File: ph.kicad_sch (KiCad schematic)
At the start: 46 parts, among them J4 Conn_01x04_Pin, J5 Conn_Coaxial, J6 Conn_01x04_Pin, U17 CA3140, U18 TL081

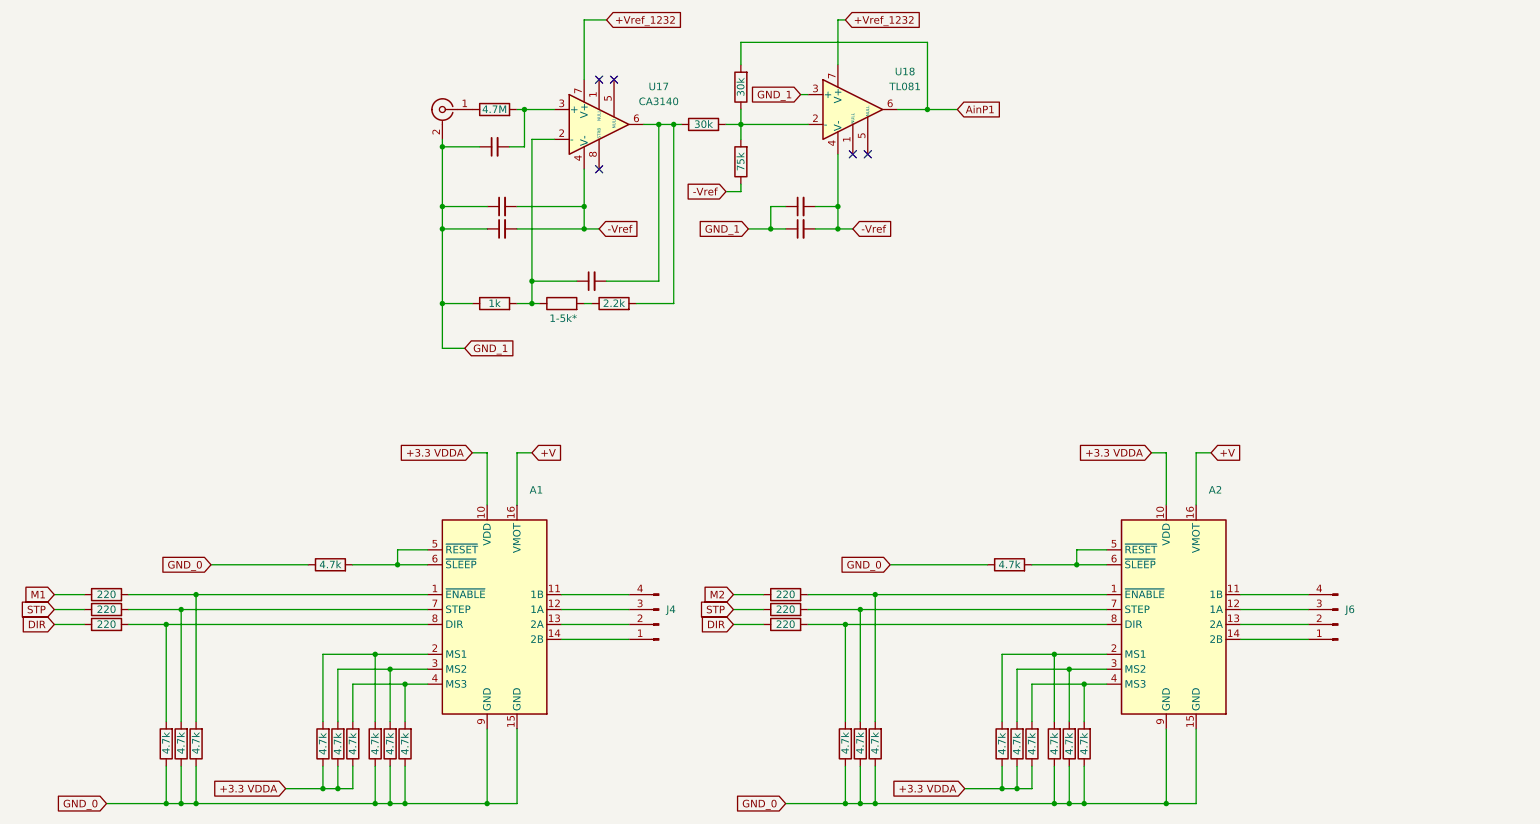
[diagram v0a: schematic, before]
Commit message: redaction_11
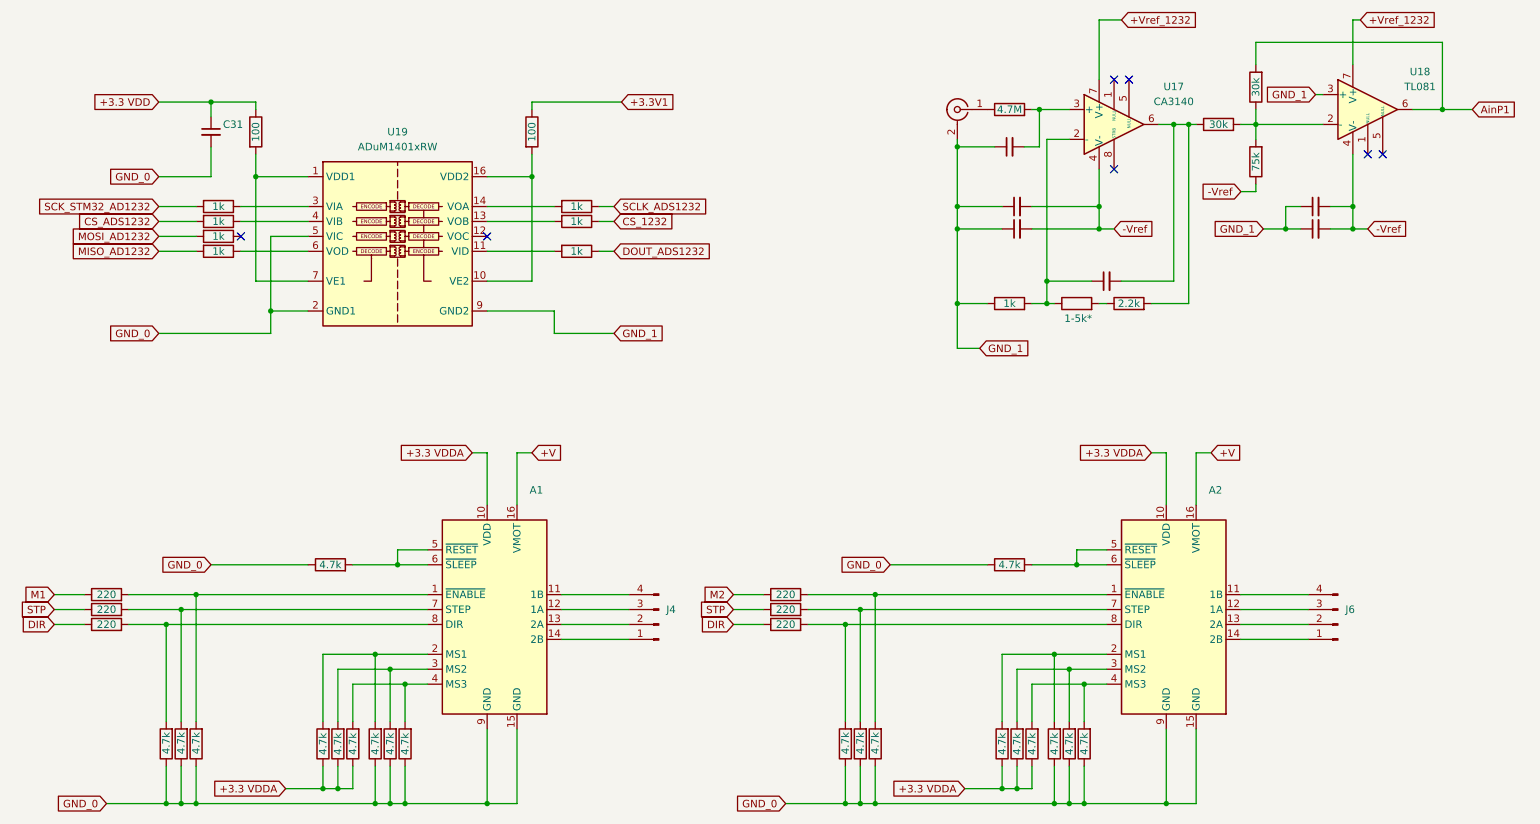
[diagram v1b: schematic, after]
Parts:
- added C31: 0.1 uF, Capacitor_SMD:C_0805_2012Metric_Pad1.18x1.45mm_HandSolder, symbol Device:C_Small
- added R106, R72: 100, Resistor_SMD:R_0805_2012Metric_Pad1.20x1.40mm_HandSolder, symbol Device:R
- added R107, R108, R109, R40, R69, R70, R71: 1k, Resistor_SMD:R_0805_2012Metric_Pad1.20x1.40mm_HandSolder, symbol Device:R
- added U19: ADuM1401xRW, Package_SO:SOIC-16W_7.5x10.3mm_P1.27mm, symbol Isolator:ADuM1401xRW
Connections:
- net GND_0: now also C31.2, U19.2 (GND1), U19.5 (VIC), U19.8 (GND1)
- net GND_1: now also U19.15 (GND2), U19.9 (GND2)
- new net: R72.2, U19.1 (VDD1), U19.7 (VE1)
- new net: R106.2, U19.10 (VE2), U19.16 (VDD2)
- new net: R108.2, U19.11 (VID)
- new net: R107.2, U19.13 (VOB)
- new net: R69.2, U19.14 (VOA)
- new net: R40.1, U19.3 (VIA)
- new net: R70.1, U19.4 (VIB)
- new net: R71.1, U19.6 (VOD)
- new net +3.3 VDD: C31.1, R72.1
- new net +3.3V1: R106.1
- new net CS_1232: R107.1
- new net CS_ADS1232: R70.2
- new net DOUT_ADS1232: R108.1
- new net MISO_AD1232: R71.2
- new net MOSI_AD1232: R109.2
- new net SCK_STM32_AD1232: R40.2
- new net SCLK_ADS1232: R69.1
- no-connect marks 5 -> 7
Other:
- moved on the sheet: U17, U18
